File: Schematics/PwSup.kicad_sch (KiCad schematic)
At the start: 32 parts, among them J3 Phase, J4 PX Ph, J5 PXB10C, J6 Neutral, J7 Px N, SW2 SW_SPST, U3 TL072, U4 LM317_TO-220

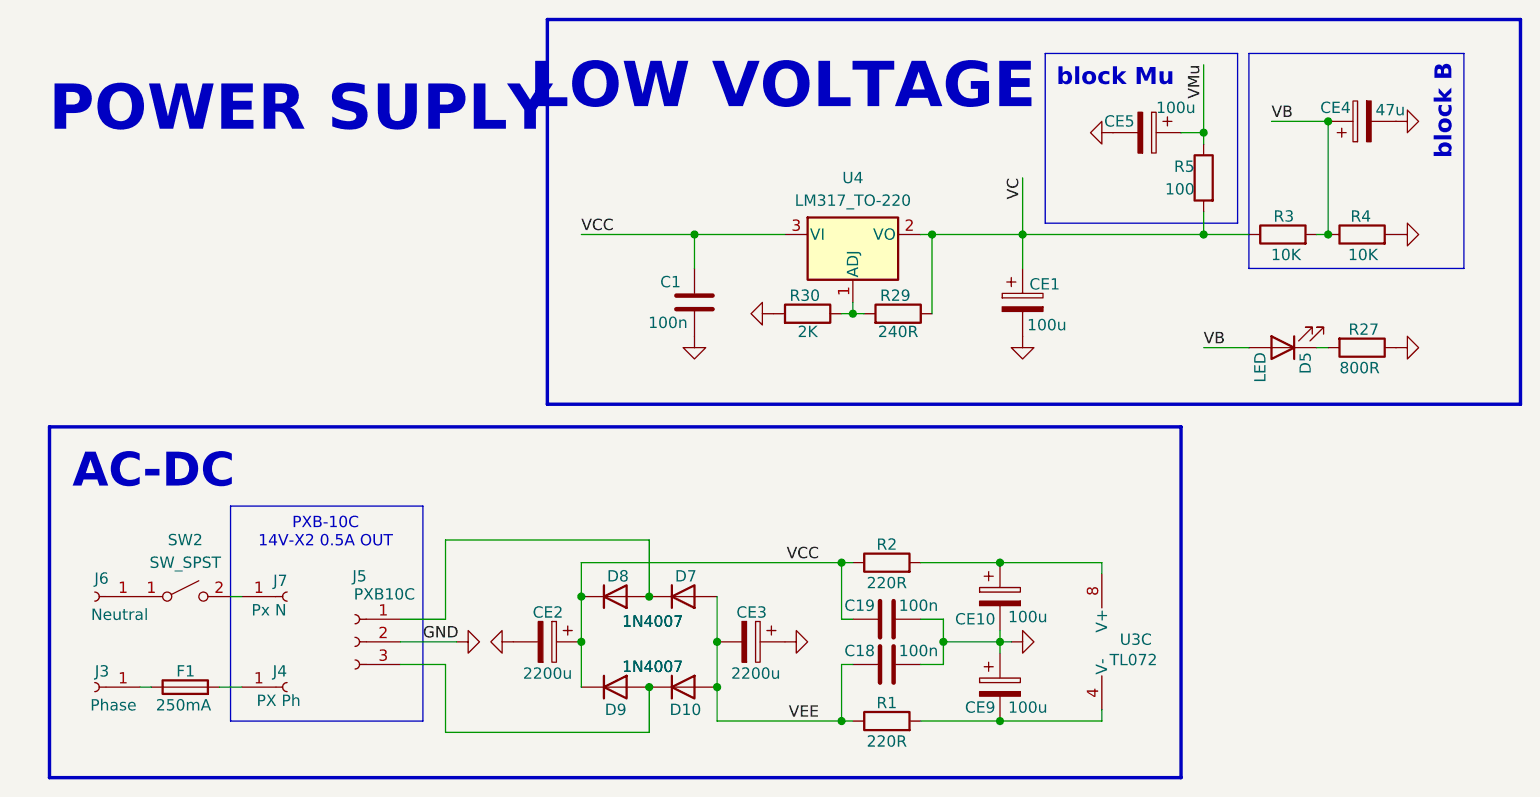
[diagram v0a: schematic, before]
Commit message: Schem upd & added .gitignore
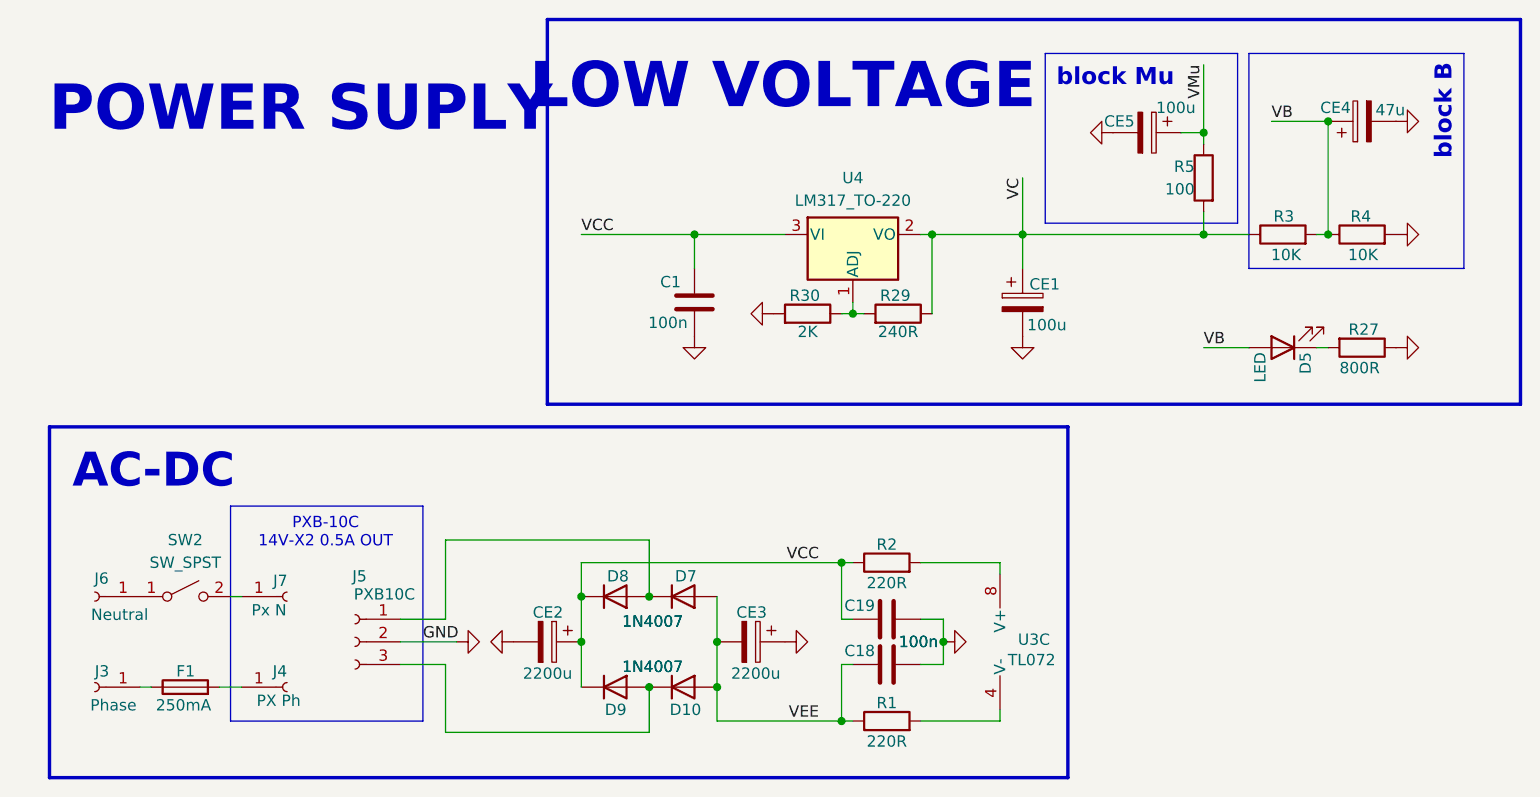
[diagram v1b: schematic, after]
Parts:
- removed CE10, CE9: 100u, Capacitor_THT:CP_Radial_D14.0mm_P7.50mm, symbol Device:C_Polarized
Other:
- moved on the sheet: U3C
